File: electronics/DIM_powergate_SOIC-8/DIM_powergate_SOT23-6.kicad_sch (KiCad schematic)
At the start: 10 parts, among them J1 Conn_01x04, J2 Conn_01x04, Q2 NMOS, Q3 Q_PMOS_DUAL

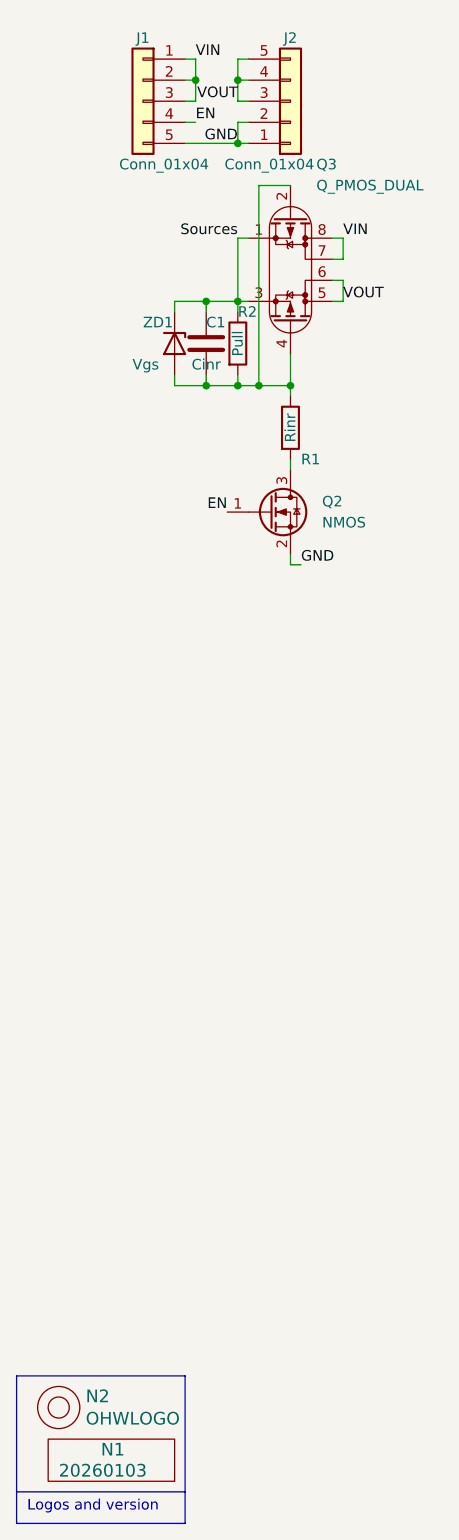
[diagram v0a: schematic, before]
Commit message: Reviewed and fixed
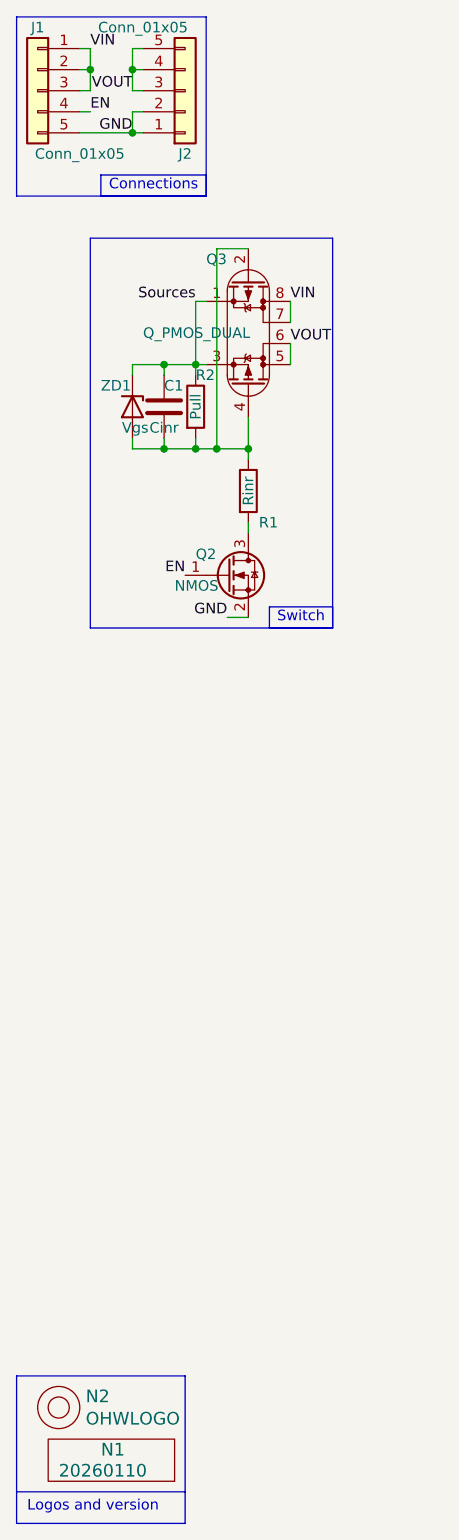
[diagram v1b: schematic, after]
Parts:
- J1, J2: value Conn_01x04 -> Conn_01x05
- N1: value 20260103 -> 20260110
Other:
- note added: "Connections"
- note added: "Switch"
- moved on the sheet: C1, J1, J2, Q2, Q3, R1, R2, ZD1
